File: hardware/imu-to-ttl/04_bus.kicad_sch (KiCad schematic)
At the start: 12 parts, among them U3 SN74LVC2G241DCUR

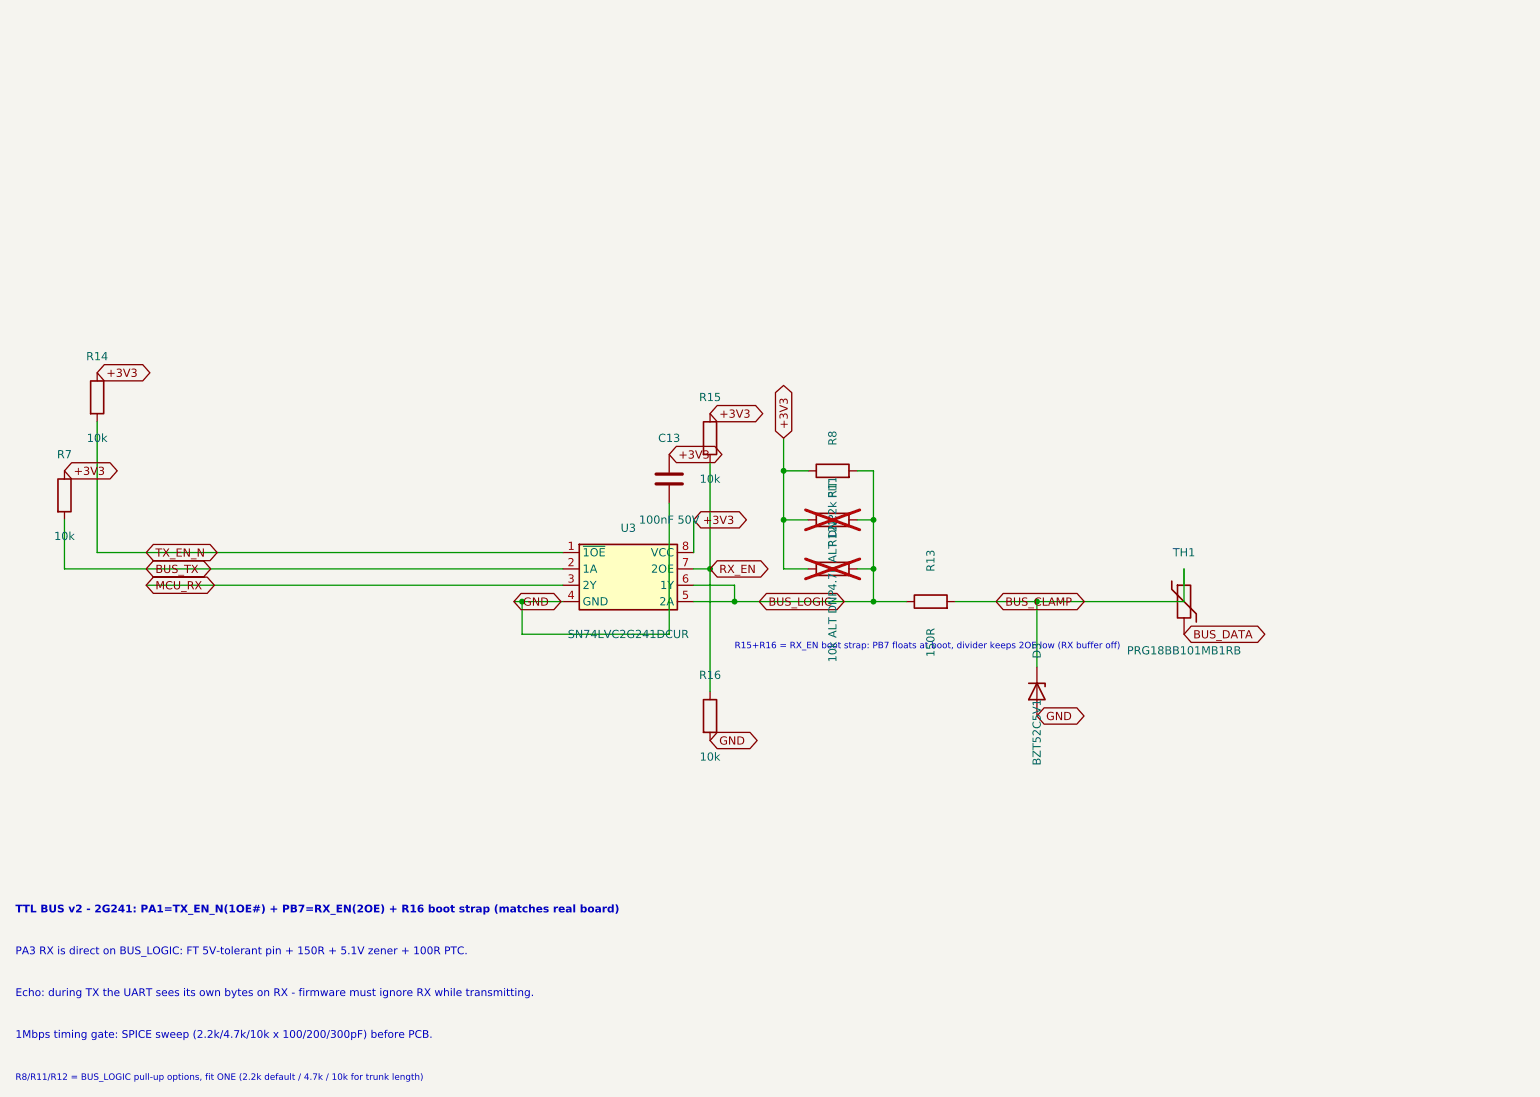
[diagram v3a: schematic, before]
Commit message: sync: 2026-10-12 日常更新
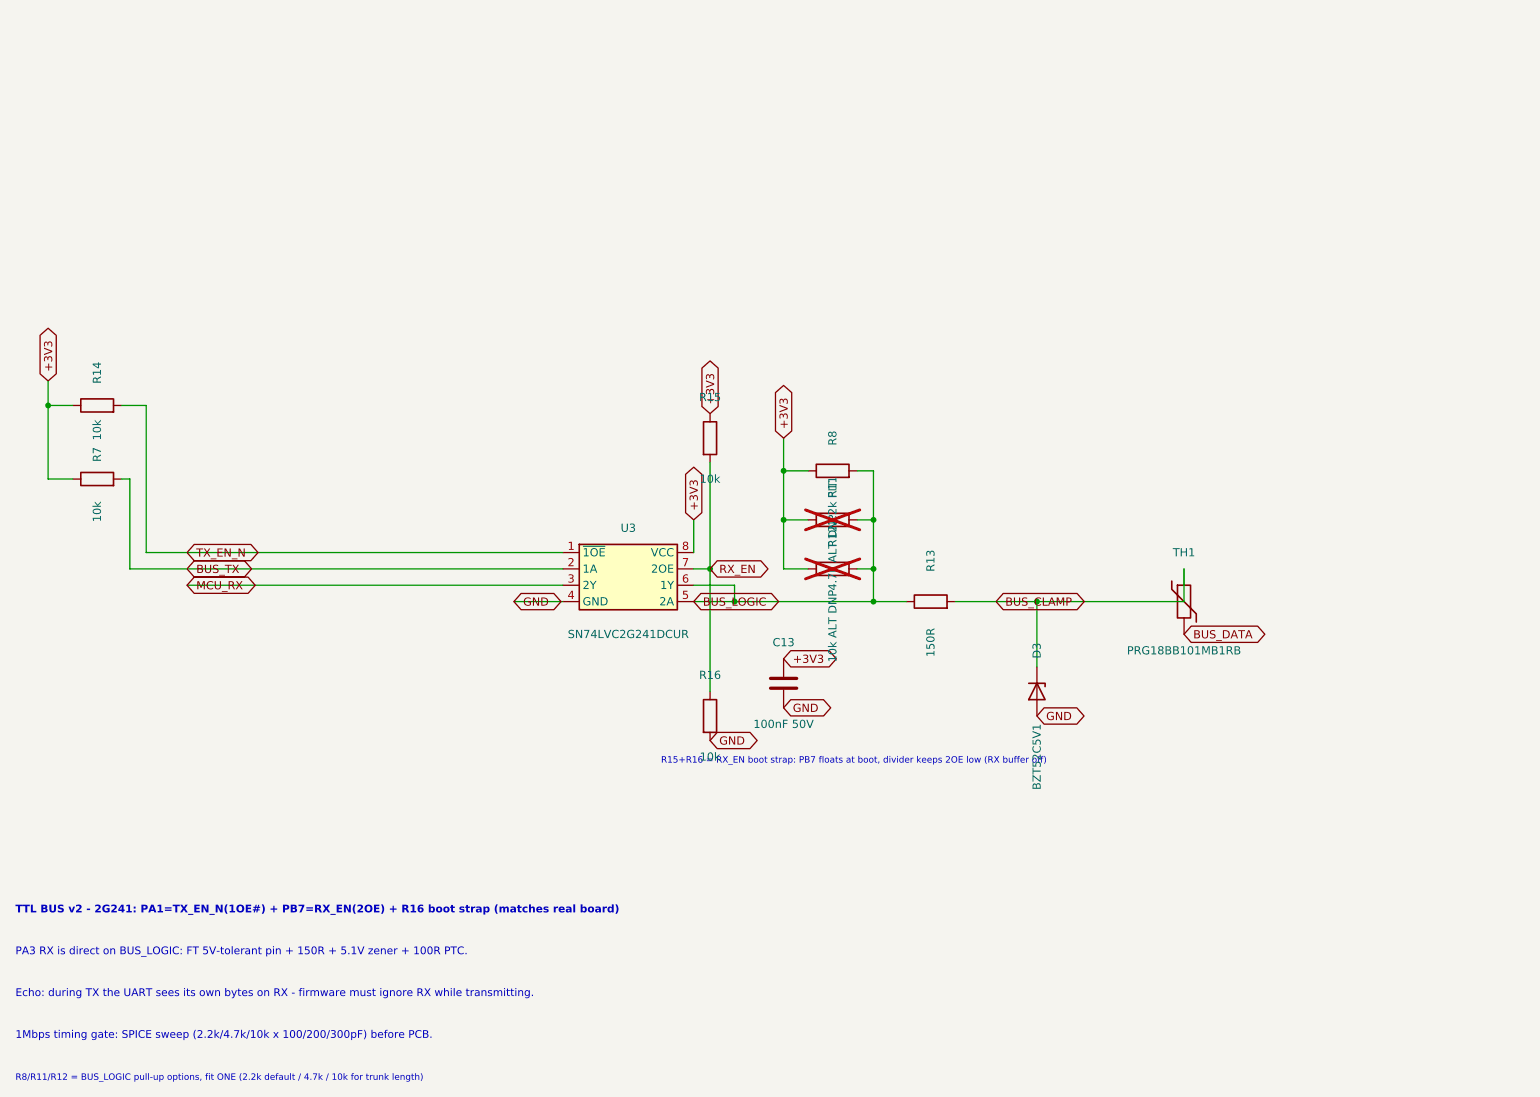
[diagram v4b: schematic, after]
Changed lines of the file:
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@@
 	(symbol
 		(lib_id "Device:R")
-		(at 38.10 82.55 0)
+		(at 38.10 83.82 90)
 		(unit 1)
 		(exclude_from_sim no)
@@
 		(dnp no)
 		(property "Reference" "R14"
-		(at 38.10 76.20 0)
+		(at 38.10 78.74 0)
 		(effects
 		(font
@@
 	)
 		(property "Value" "10k"
-		(at 38.10 88.90 0)
+		(at 38.10 87.63 0)
 		(effects
 		(font
@@
 	(symbol
 		(lib_id "Device:R")
-		(at 33.02 97.79 0)
+		(at 38.10 95.25 90)
 		(unit 1)
 		(exclude_from_sim no)
@@
 		(dnp no)
 		(property "Reference" "R7"
-		(at 33.02 91.44 0)
+		(at 38.10 91.44 0)
 		(effects
 		(font
@@
 	)
 		(property "Value" "10k"
-		(at 33.02 104.14 0)
+		(at 38.10 100.33 0)
 		(effects
 		(font
@@
 	)
 		(property "Value" "BZT52C5V1"
-		(at 184.15 134.62 0)
+		(at 184.15 138.43 0)
 		(effects
 		(font
@@
 	(symbol
 		(lib_id "Device:C")
-		(at 127.00 95.25 0)
+		(at 144.78 127.00 0)
 		(unit 1)
 		(exclude_from_sim no)
@@
 		(dnp no)
 		(property "Reference" "C13"
-		(at 127.00 88.90 0)
+		(at 144.78 120.65 0)
 		(effects
 		(font
@@
 	)
 		(property "Value" "100nF 50V"
-		(at 127.00 101.60 0)
+		(at 144.78 133.35 0)
 		(effects
 		(font
@@
 	)
 	(wire
-		(pts (xy 38.10 86.36) (xy 38.10 106.68))
-		(stroke
-			(width 0)
-			(type default)
-		)
-	)
-	(wire
-		(pts (xy 38.10 106.68) (xy 110.49 106.68))
-		(stroke
-			(width 0)
-			(type default)
-		)
-	)
-	(wire
-		(pts (xy 33.02 101.60) (xy 33.02 109.22))
-		(stroke
-			(width 0)
-			(type default)
-		)
-	)
-	(wire
-		(pts (xy 33.02 109.22) (xy 110.49 109.22))
-		(stroke
-			(width 0)
-			(type default)
-		)
-	)
-	(wire
-		(pts (xy 45.72 111.76) (xy 110.49 111.76))
+		(pts (xy 30.48 80.01) (xy 30.48 95.25))
+		(stroke
+			(width 0)
+			(type default)
+		)
+	)
+	(wire
+		(pts (xy 30.48 83.82) (xy 34.29 83.82))
+		(stroke
+			(width 0)
+			(type default)
+		)
+	)
+	(wire
+		(pts (xy 41.91 83.82) (xy 45.72 83.82))
+		(stroke
+			(width 0)
+			(type default)
+		)
+	)
+	(wire
+		(pts (xy 45.72 83.82) (xy 45.72 106.68))
+		(stroke
+			(width 0)
+			(type default)
+		)
+	)
+	(wire
+		(pts (xy 30.48 95.25) (xy 34.29 95.25))
+		(stroke
+			(width 0)
+			(type default)
+		)
+	)
+	(wire
+		(pts (xy 41.91 95.25) (xy 43.18 95.25))
+		(stroke
+			(width 0)
+			(type default)
+		)
+	)
+	(wire
+		(pts (xy 43.18 95.25) (xy 43.18 109.22))
+		(stroke
+			(width 0)
+			(type default)
+		)
+	)
+	(wire
+		(pts (xy 45.72 106.68) (xy 110.49 106.68))
+		(stroke
+			(width 0)
+			(type default)
+		)
+	)
+	(wire
+		(pts (xy 43.18 109.22) (xy 110.49 109.22))
+		(stroke
+			(width 0)
+			(type default)
+		)
+	)
+	(wire
+		(pts (xy 52.07 111.76) (xy 110.49 111.76))
 		(stroke
 			(width 0)
@@
 	)
 	(wire
-		(pts (xy 127.00 99.06) (xy 127.00 119.38))
-		(stroke
-			(width 0)
-			(type default)
-		)
-	)
-	(wire
-		(pts (xy 127.00 119.38) (xy 104.14 119.38))
-		(stroke
-			(width 0)
-			(type default)
-		)
-	)
-	(wire
-		(pts (xy 104.14 119.38) (xy 104.14 114.30))
-		(stroke
-			(width 0)
-			(type default)
-		)
-	)
-	(wire
 		(pts (xy 184.15 114.30) (xy 184.15 124.46))
 		(stroke
@@
 		)
 	)
+	(junction (at 30.48 83.82) (diameter 0) (color 0 0 0 0)
+	)
 	(junction (at 133.35 109.22) (diameter 0) (color 0 0 0 0)
 	)
@@
 	(junction (at 158.75 109.22) (diameter 0) (color 0 0 0 0)
 	)
-	(junction (at 104.14 114.30) (diameter 0) (color 0 0 0 0)
-	)
 	(global_label "TX_EN_N"
 		(shape bidirectional)
-		(at 45.72 106.68 0)
+		(at 52.07 106.68 0)
 		(fields_autoplaced yes)
 		(effects
@@
 	(global_label "BUS_TX"
 		(shape bidirectional)
-		(at 45.72 109.22 0)
+		(at 52.07 109.22 0)
 		(fields_autoplaced yes)
 		(effects
@@
 	(global_label "MCU_RX"
 		(shape bidirectional)
-		(at 45.72 111.76 0)
+		(at 52.07 111.76 0)
 		(fields_autoplaced yes)
 		(effects
@@
 	(global_label "+3V3"
 		(shape bidirectional)
-		(at 38.10 78.74 0)
+		(at 30.48 80.01 90)
 		(fields_autoplaced yes)
 		(effects
@@
 	(global_label "+3V3"
 		(shape bidirectional)
-		(at 33.02 93.98 0)
+		(at 130.81 101.60 90)
 		(fields_autoplaced yes)
 		(effects
@@
 	(global_label "+3V3"
 		(shape bidirectional)
-		(at 130.81 101.60 0)
+		(at 133.35 85.09 90)
+		(fields_autoplaced yes)
+		(effects
+			(font (size 1.27 1.27)) (justify left)
+		)
+	)
+	(global_label "RX_EN"
+		(shape bidirectional)
+		(at 133.35 109.22 0)
+		(fields_autoplaced yes)
+		(effects
+			(font (size 1.27 1.27)) (justify left)
+		)
+	)
+	(global_label "GND"
+		(shape bidirectional)
+		(at 133.35 135.89 0)
 		(fields_autoplaced yes)
 		(effects
@@
 	(global_label "+3V3"
 		(shape bidirectional)
-		(at 133.35 85.09 0)
-		(fields_autoplaced yes)
-		(effects
-			(font (size 1.27 1.27)) (justify left)
-		)
-	)
-	(global_label "RX_EN"
-		(shape bidirectional)
-		(at 133.35 109.22 0)
+		(at 144.78 88.90 90)
+		(fields_autoplaced yes)
+		(effects
+			(font (size 1.27 1.27)) (justify left)
+		)
+	)
+	(global_label "BUS_LOGIC"
+		(shape bidirectional)
+		(at 130.81 114.30 0)
+		(fields_autoplaced yes)
+		(effects
+			(font (size 1.27 1.27)) (justify left)
+		)
+	)
+	(global_label "BUS_CLAMP"
+		(shape bidirectional)
+		(at 177.80 114.30 0)
 		(fields_autoplaced yes)
 		(effects
@@
 	(global_label "GND"
 		(shape bidirectional)
-		(at 133.35 135.89 0)
+		(at 184.15 132.08 0)
+		(fields_autoplaced yes)
+		(effects
+			(font (size 1.27 1.27)) (justify left)
+		)
+	)
+	(global_label "BUS_DATA"
+		(shape bidirectional)
+		(at 207.01 119.38 0)
 		(fields_autoplaced yes)
 		(effects
@@
 	(global_label "+3V3"
 		(shape bidirectional)
-		(at 144.78 88.90 90)
-		(fields_autoplaced yes)
-		(effects
-			(font (size 1.27 1.27)) (justify left)
-		)
-	)
-	(global_label "BUS_LOGIC"
-		(shape bidirectional)
-		(at 141.00 114.30 0)
-		(fields_autoplaced yes)
-		(effects
-			(font (size 1.27 1.27)) (justify left)
-		)
-	)
-	(global_label "BUS_CLAMP"
-		(shape bidirectional)
-		(at 177.80 114.30 0)
+		(at 144.78 123.19 0)
 		(fields_autoplaced yes)
 		(effects
@@
 	(global_label "GND"
 		(shape bidirectional)
-		(at 184.15 132.08 0)
-		(fields_autoplaced yes)
-		(effects
-			(font (size 1.27 1.27)) (justify left)
-		)
-	)
-	(global_label "BUS_DATA"
-		(shape bidirectional)
-		(at 207.01 119.38 0)
-		(fields_autoplaced yes)
-		(effects
-			(font (size 1.27 1.27)) (justify left)
-		)
-	)
-	(global_label "+3V3"
-		(shape bidirectional)
-		(at 127.00 91.44 0)
+		(at 144.78 130.81 0)
 		(fields_autoplaced yes)
 		(effects
@@
 	)
 	(text "R15+R16 = RX_EN boot strap: PB7 floats at boot, divider keeps 2OE low (RX buffer off)"
-		(at 137.16 121.92 0)
+		(at 125.73 139.70 0)
 		(effects (font (size 1 1)) (justify left bottom))
 	)

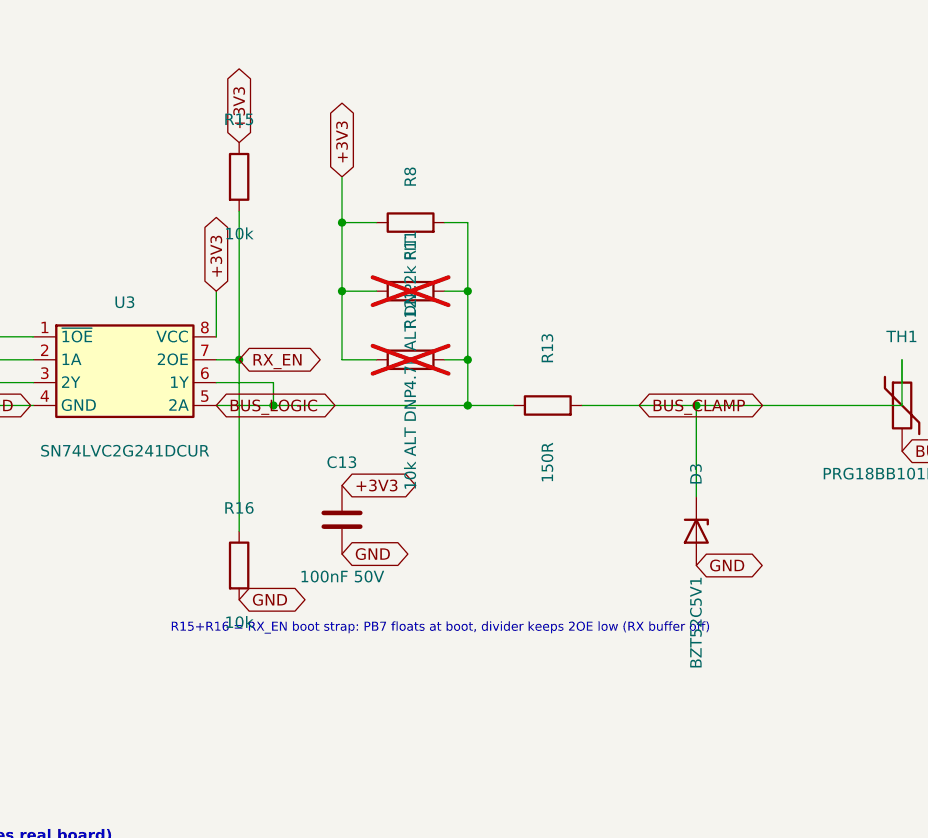
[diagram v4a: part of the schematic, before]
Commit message: sync: 2026-10-12 日常更新
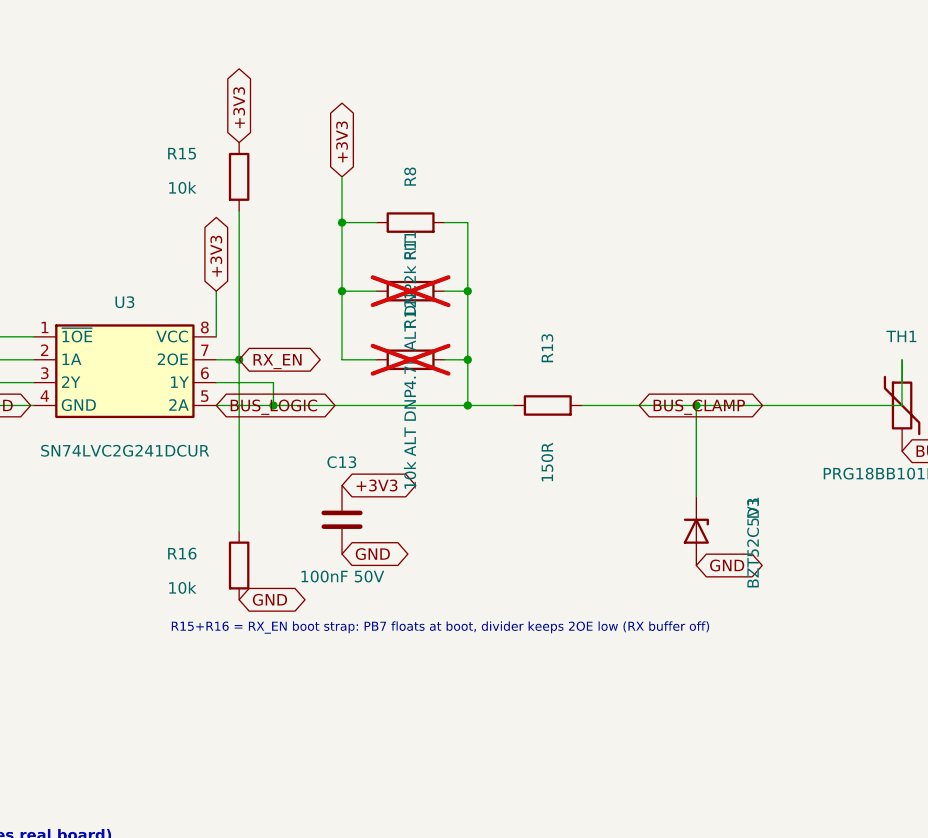
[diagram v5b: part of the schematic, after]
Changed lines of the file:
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@@
 		(dnp no)
 		(property "Reference" "R15"
-		(at 133.35 82.55 0)
+		(at 127.00 86.36 0)
 		(effects
 		(font
@@
 	)
 		(property "Value" "10k"
-		(at 133.35 95.25 0)
+		(at 127.00 90.17 0)
 		(effects
 		(font
@@
 		(dnp no)
 		(property "Reference" "R16"
-		(at 133.35 125.73 0)
+		(at 127.00 130.81 0)
 		(effects
 		(font
@@
 	)
 		(property "Value" "10k"
-		(at 133.35 138.43 0)
+		(at 127.00 134.62 0)
 		(effects
 		(font
@@
 		(dnp no)
 		(property "Reference" "D3"
-		(at 184.15 121.92 0)
+		(at 190.50 125.73 0)
 		(effects
 		(font
@@
 	)
 		(property "Value" "BZT52C5V1"
-		(at 184.15 138.43 0)
-		(effects
-		(font
+		(at 190.50 129.54 0)
+		(effects
+		(font
